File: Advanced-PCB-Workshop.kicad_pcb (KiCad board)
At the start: 4 copper layers, 39.9 x 39.5 mm, 36 parts, among them J1 USB_C_Receptacle_USB2.0_14P, J2 Conn_01x03_Pin, J3 Conn_01x14_Socket, J4 Conn_01x14_Socket, SW1 SW_Nidec_CAS-120A1, SW2 SW_Push, U1 RP2040, U2 W25Q128JVS, U3 AMS1117-3.3, Y1 ABM8-272-T3

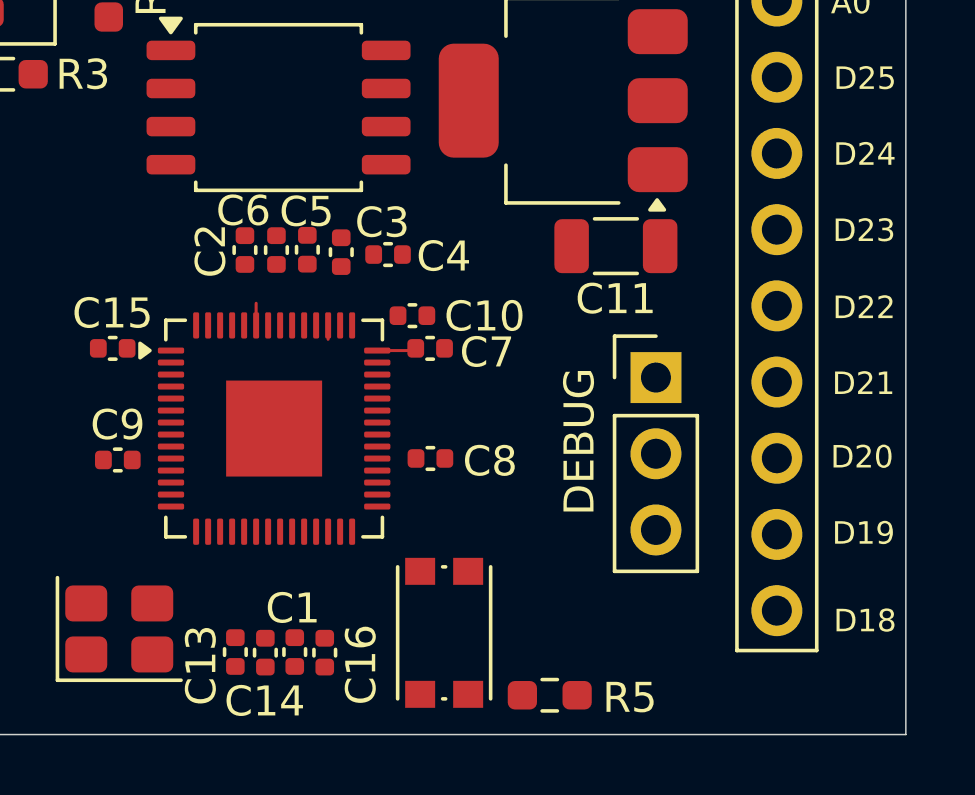
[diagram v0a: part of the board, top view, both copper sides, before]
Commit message: Finish Template Board
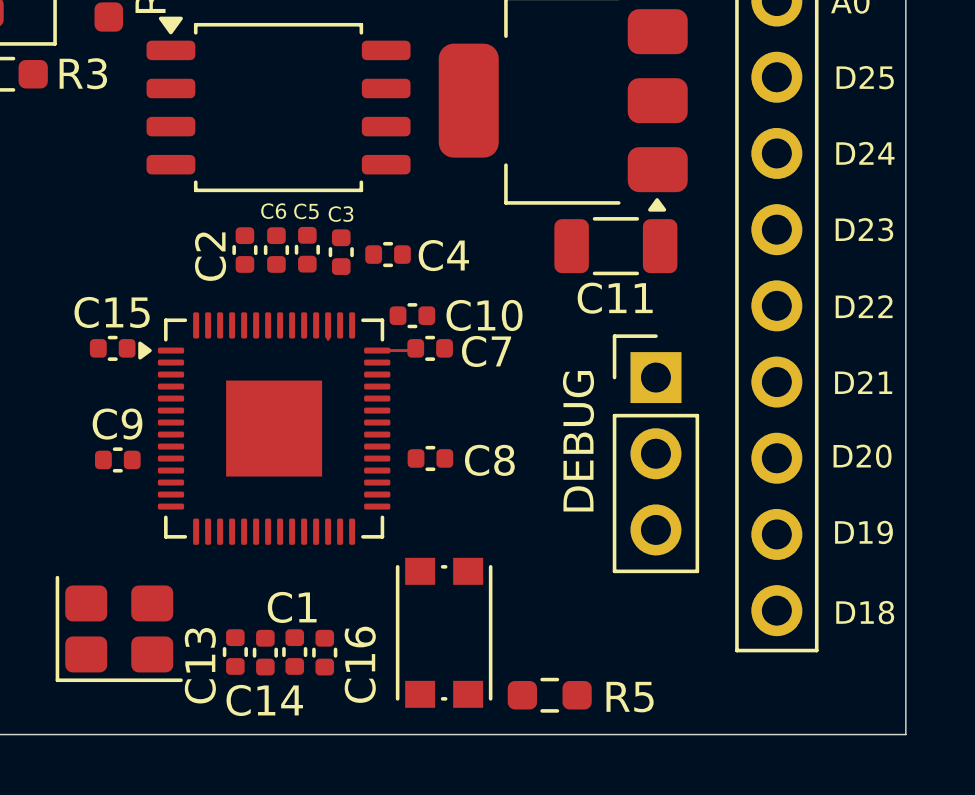
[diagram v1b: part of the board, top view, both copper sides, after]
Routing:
- net QSPI_SD3: track 1.41 -> 0.67 mm
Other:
- copper layers 4 -> 2
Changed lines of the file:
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@@
 	(layers
 		(0 "F.Cu" signal)
-		(4 "In1.Cu" signal)
-		(6 "In2.Cu" signal)
 		(2 "B.Cu" signal)
 		(9 "F.Adhes" user "F.Adhesive")
@@
 			)
 			(layer "dielectric 1"
-				(type "prepreg")
-				(thickness 0.1)
-				(material "FR4")
-				(epsilon_r 4.5)
-				(loss_tangent 0.02)
-			)
-			(layer "In1.Cu"
-				(type "copper")
-				(thickness 0.035)
-			)
-			(layer "dielectric 2"
 				(type "core")
-				(thickness 1.24)
-				(material "FR4")
-				(epsilon_r 4.5)
-				(loss_tangent 0.02)
-			)
-			(layer "In2.Cu"
-				(type "copper")
-				(thickness 0.035)
-			)
-			(layer "dielectric 3"
-				(type "prepreg")
-				(thickness 0.1)
+				(thickness 1.51)
 				(material "FR4")
 				(epsilon_r 4.5)
@@
 		(tags "capacitor")
 		(property "Reference" "C3"
-			(at -0.98 -1.37 0)
+			(at -1.25 0 0)
 			(layer "F.SilkS")
 			(effects
 				(font
-					(size 1 1)
-					(thickness 0.15)
+					(size 0.5 0.5)
+					(thickness 0.125)
 				)
 			)
@@
 		(tags "capacitor")
 		(property "Reference" "C6"
-			(at -1.3 1.1 180)
+			(at -1.28 0.09 180)
 			(layer "F.SilkS")
 			(effects
 				(font
-					(size 1 1)
-					(thickness 0.15)
+					(size 0.5 0.5)
+					(thickness 0.125)
 				)
 			)
@@
 			(effects
 				(font
-					(size 1 1)
-					(thickness 0.15)
+					(size 0.5 0.5)
+					(thickness 0.125)
 				)
 			)
@@
 		(tags "capacitor")
 		(property "Reference" "C2"
-			(at 0.02 1.13 90)
+			(at 0.19 1.11 90)
 			(layer "F.SilkS")
 			(effects
@@
 	)
 	(gr_text "D18"
-		(at 150.62 118.14 0)
+		(at 150.61 117.89 0)
 		(layer "F.SilkS")
 		(effects
@@
 		(width 0.1)
 		(layer "F.Cu")
-		(net 48)
-	)
-	(segment
-		(start 131.3725 107.8525)
-		(end 131.3725 107.1125)
-		(width 0.1)
-		(layer "F.Cu")
